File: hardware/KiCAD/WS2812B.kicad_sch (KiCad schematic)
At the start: 2 parts, among them U11 74AHCT1G125

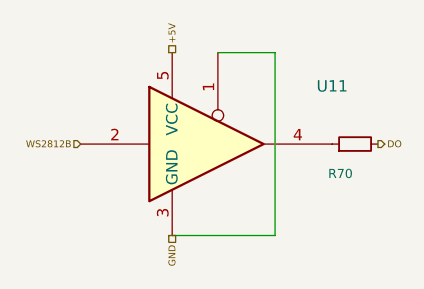
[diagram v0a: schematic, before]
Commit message: update
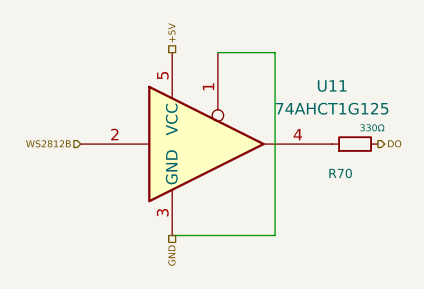
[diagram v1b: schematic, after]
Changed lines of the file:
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@@
 					(size 1.27 1.27)
 				)
-				(hide yes)
 			)
 		)
@@
 				)
 				(justify left)
-				(hide yes)
 			)
 		)

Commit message: update
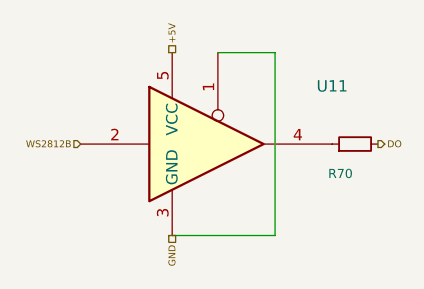
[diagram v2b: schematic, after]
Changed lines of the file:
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@@
 					(size 1.27 1.27)
 				)
+				(hide yes)
 			)
 		)
@@
 				)
 				(justify left)
+				(hide yes)
 			)
 		)
